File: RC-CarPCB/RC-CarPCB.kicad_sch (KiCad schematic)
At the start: 13 parts, among them J1 Conn_01x02_Pin, SW1 SW_SPST, SW2 SW_SPST, SW3 SW_SPST, SW4 SW_SPST, U1 NRF24L01_Breakout

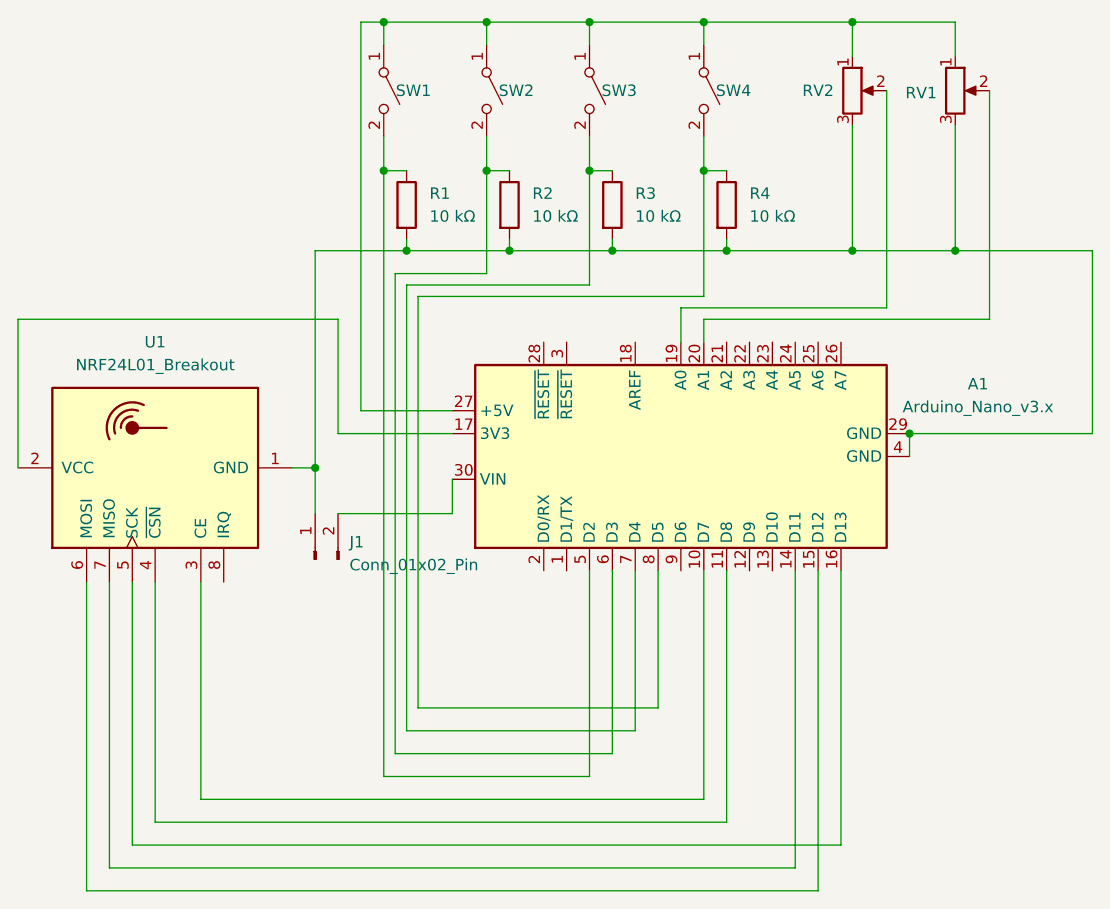
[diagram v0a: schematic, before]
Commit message: stuff
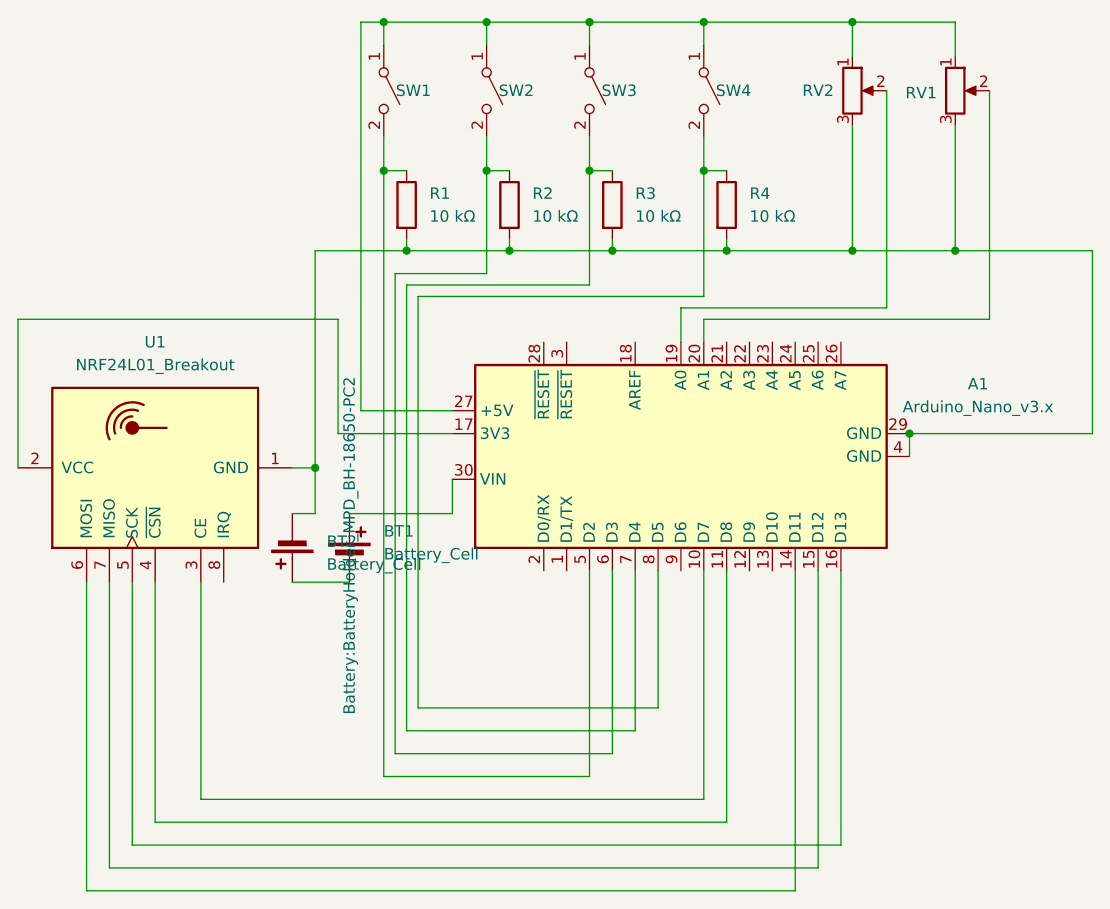
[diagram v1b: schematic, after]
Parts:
- removed J1: Conn_01x02_Pin, Connector:JWT_A3963_1x02_P3.96mm_Vertical, symbol Connector:Conn_01x02_Pin
- added BT1, BT2: Battery_Cell, Battery:BatteryHolder_MPD_BH-18650-PC2, symbol Device:Battery_Cell
- RV1, RV2: footprint Potentiometer_THT:Potentiometer_Bourns_PTA6043_Single_Slide -> CustomElements:PotentiometerSlider88mm
- SW1, SW2, SW3, SW4: footprint Button_Switch_SMD:SW_SPST_PTS647_Sx50 -> Button_Switch_THT:SW_PUSH_6mm
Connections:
- net at A1.29 (GND), A1.4 (GND), R1.2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: now also BT2.2 (-)
- net at A1.30 (VIN): now also BT1.1 (+)
- net at U1.6 (MOSI): now also A1.14 (D11); no longer A1.15 (D12)
- net at U1.7 (MISO): now also A1.15 (D12); no longer A1.14 (D11)
- new net: BT1.2 (-), BT2.1 (+)
